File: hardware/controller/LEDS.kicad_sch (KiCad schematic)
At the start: 21 parts, among them IC901 PCA9685PW_Q900,118, Q901 IRLML6402TRPBF, Q902 IRLML6402TRPBF

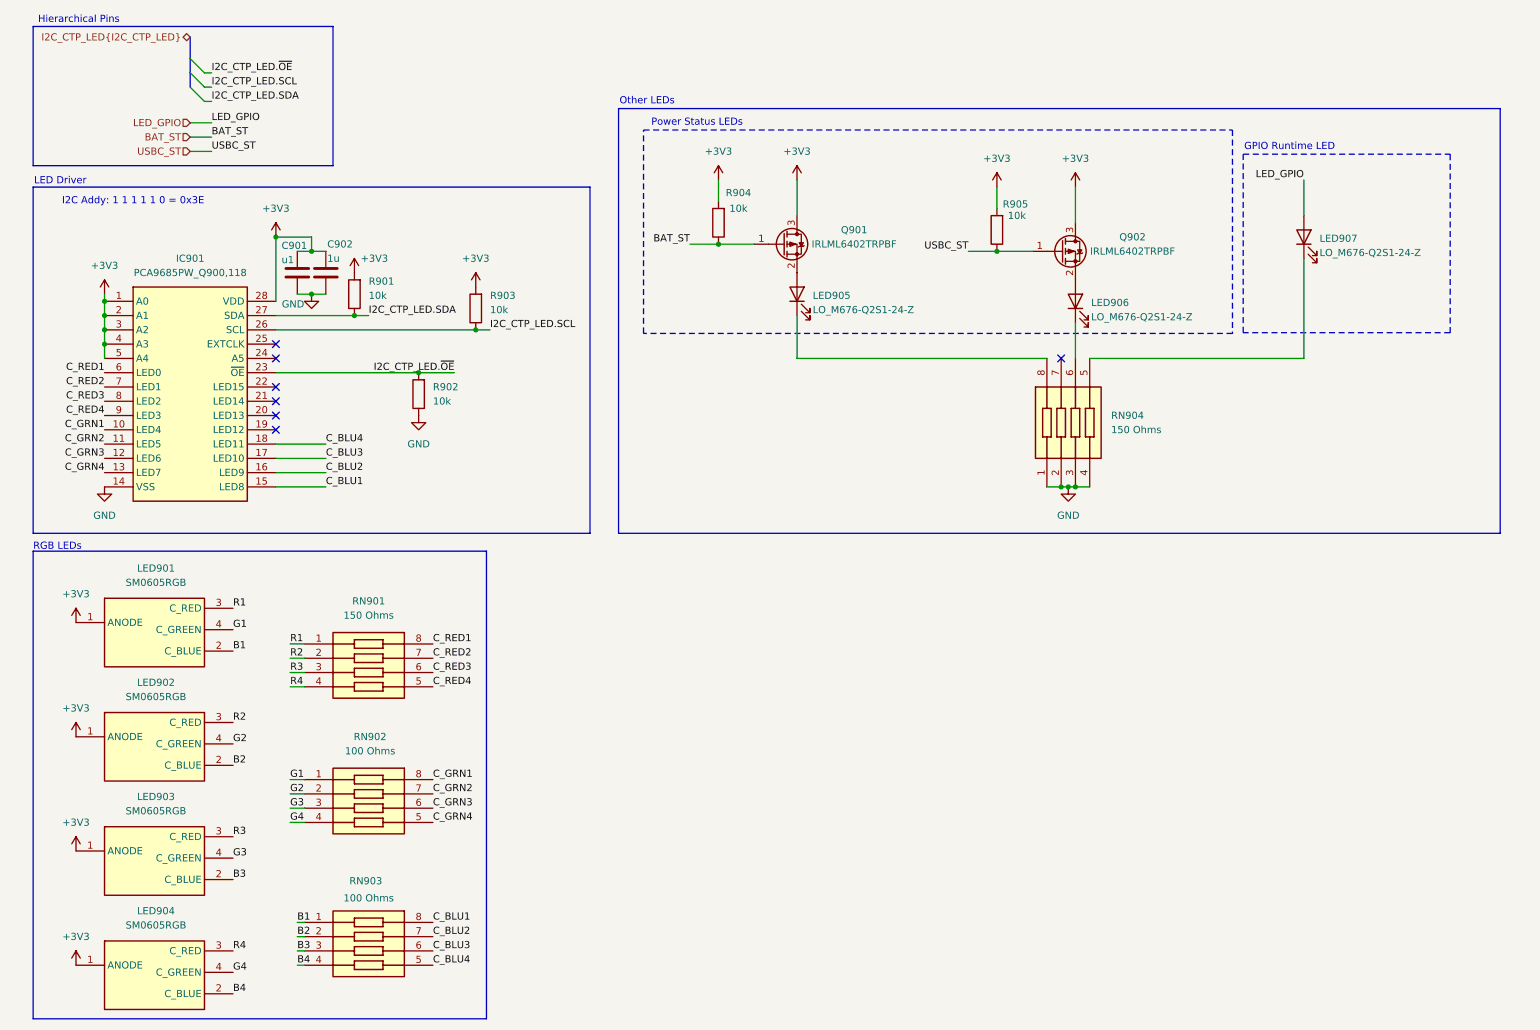
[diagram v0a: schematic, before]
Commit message: a
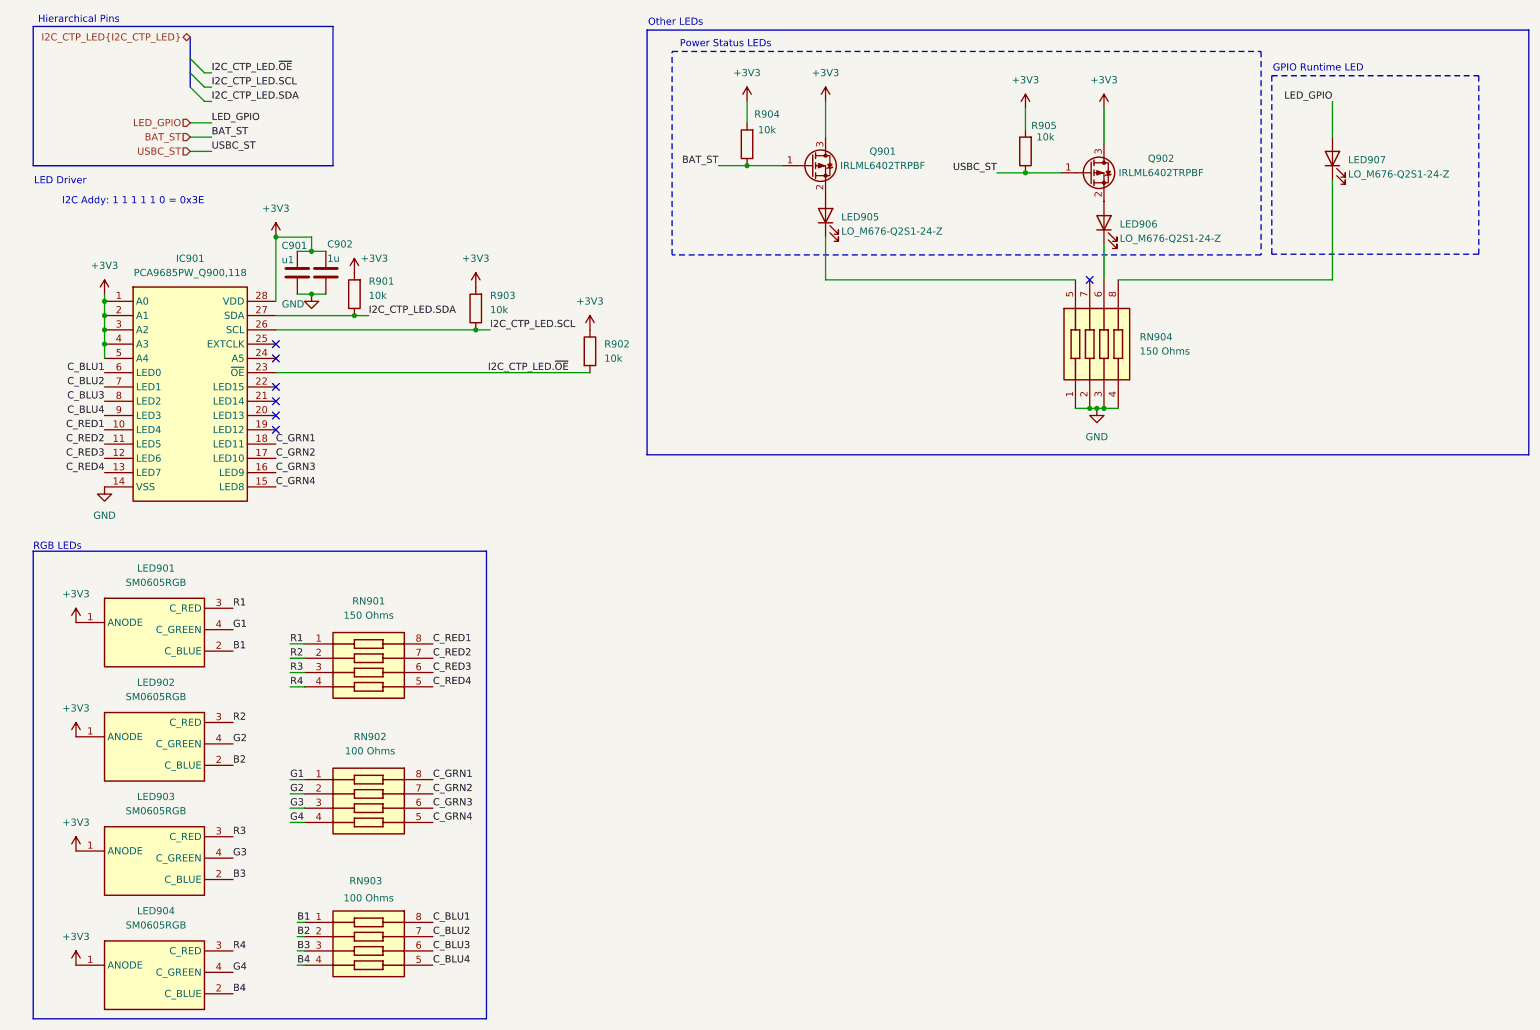
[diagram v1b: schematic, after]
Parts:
- R901, R902, R903, R904, R905: footprint SamacSys_Parts:RESC2012X60N -> RESC2012X60N
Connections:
- net +3V3: now also R902.1
- net C_BLU1: now also IC901.6 (LED0); no longer IC901.15 (LED8)
- net C_BLU2: now also IC901.7 (LED1); no longer IC901.16 (LED9)
- net C_BLU3: now also IC901.8 (LED2); no longer IC901.17 (LED10)
- net C_BLU4: now also IC901.9 (LED3); no longer IC901.18 (LED11)
- net C_GRN1: now also IC901.18 (LED11); no longer IC901.10 (LED4)
- net C_GRN2: now also IC901.17 (LED10); no longer IC901.11 (LED5)
- net C_GRN3: now also IC901.16 (LED9); no longer IC901.12 (LED6)
- net C_GRN4: now also IC901.15 (LED8); no longer IC901.13 (LED7)
- net C_RED1: now also IC901.10 (LED4); no longer IC901.6 (LED0)
- net C_RED2: now also IC901.11 (LED5); no longer IC901.7 (LED1)
- net C_RED3: now also IC901.12 (LED6); no longer IC901.8 (LED2)
- net C_RED4: now also IC901.13 (LED7); no longer IC901.9 (LED3)
- net GND: no longer R902.1
- net at LED907.1 (K): now also RN904.8; no longer RN904.5
- net at LED905.1 (K): now also RN904.5; no longer RN904.8
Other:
- moved on the sheet: LED905, LED906, LED907, Q901, Q902, R902, R904, R905, RN904
